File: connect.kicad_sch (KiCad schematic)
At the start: 18 parts, among them J10 USB_A, J11 Conn_01x02, J16 Debug, J9 USB_OTG, U10 AP22653W6-7, U11 TPD4EUSB30

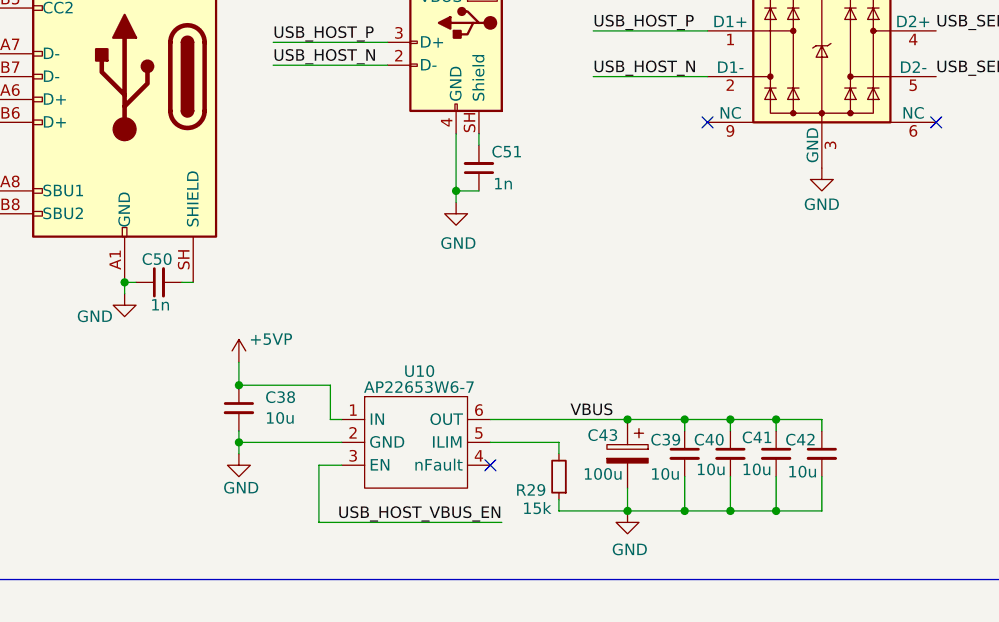
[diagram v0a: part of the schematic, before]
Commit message: fixed warnings.
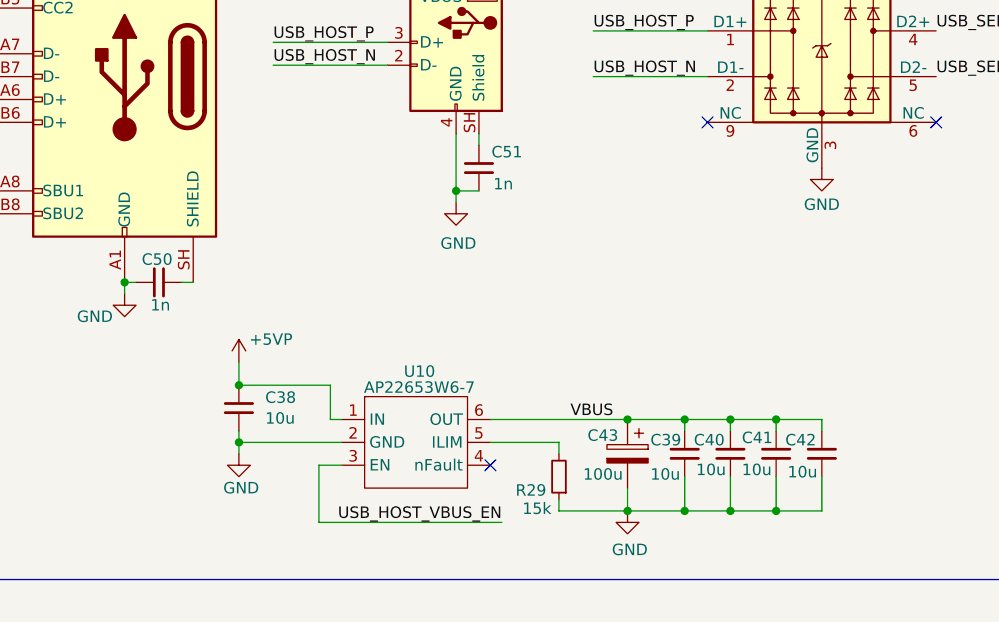
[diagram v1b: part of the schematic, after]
